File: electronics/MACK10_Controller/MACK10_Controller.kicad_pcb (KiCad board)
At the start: 2 copper layers, 97.4 x 100.5 mm, 31 parts, among them J1 Stepper Motor, J10 I/O, J3 Load Cell, J4 24V IN, J5 SSD1306, J6 INPUT, J7 E_STOP, J8 LIM_TOP, J9 LIM_BOT, U1 U1 ESP32_DEVKIT_30P, U2 HX711, U3 TMC2208, U4 LM2596 Buck Converter

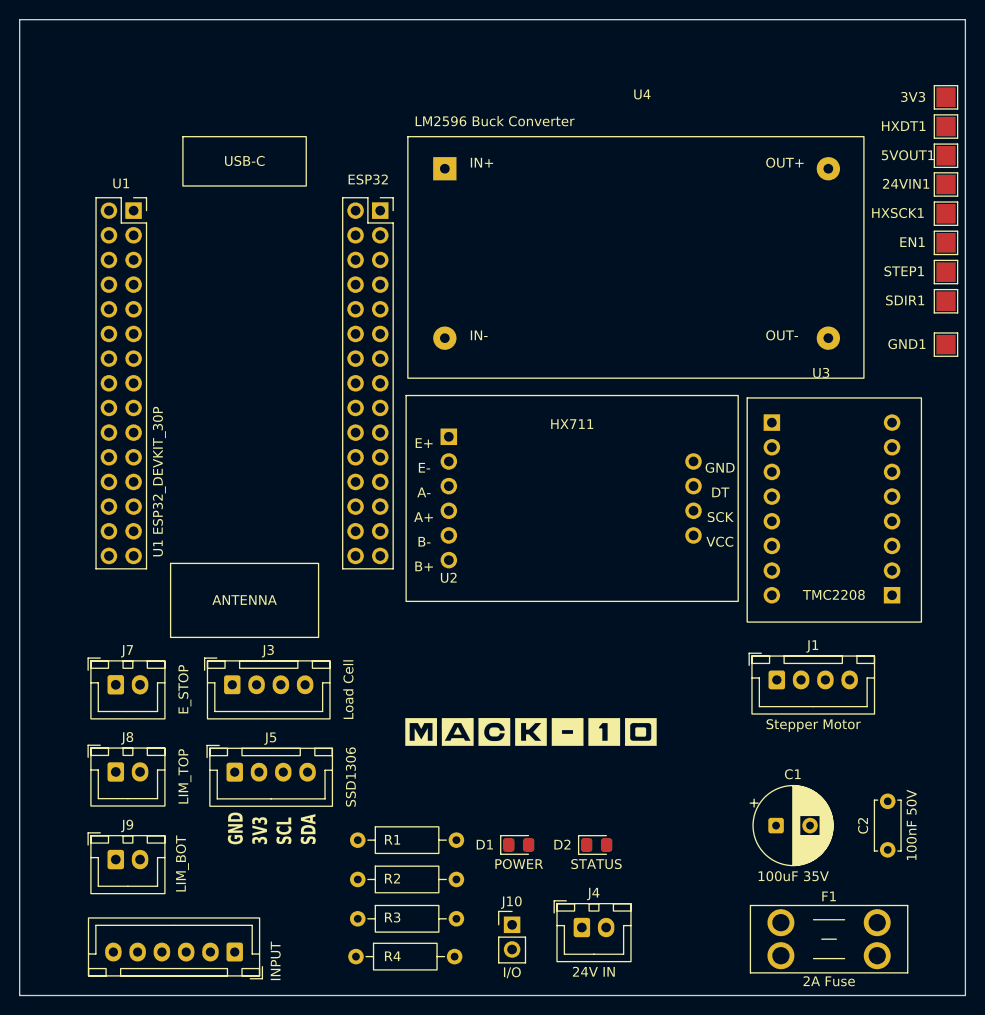
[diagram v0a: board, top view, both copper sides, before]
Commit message: Add Todo and various PCB updates
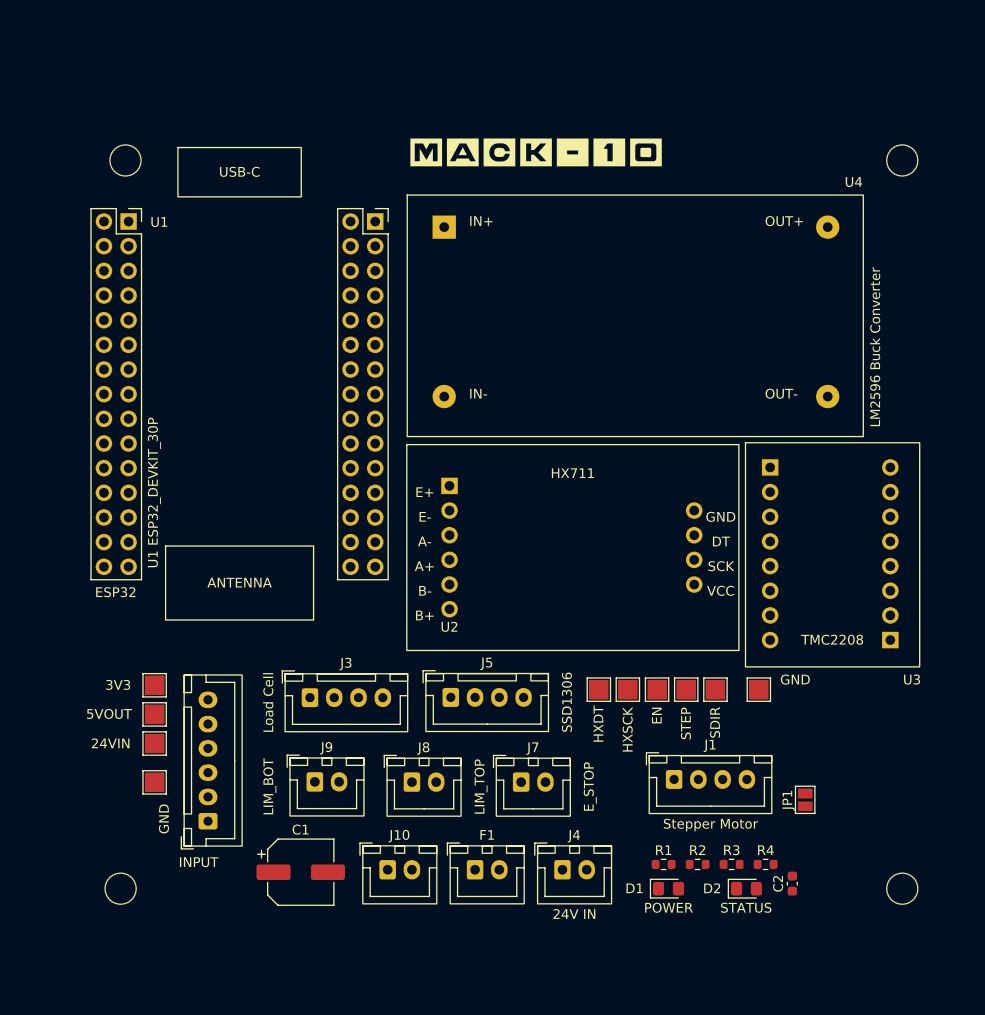
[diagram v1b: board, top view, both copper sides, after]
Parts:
- added JP1: FUSE_BYPASS, Jumper:SolderJumper-2_P1.3mm_Open_Pad1.0x1.5mm, F.Cu at (95.0, 90.8)
- added REF**: MountingHole_3.2mm_M3, MountingHole:MountingHole_3.2mm_M3, F.Cu at (25.0, 25.0)
- added REF**: MountingHole_3.2mm_M3, MountingHole:MountingHole_3.2mm_M3, F.Cu at (105.0, 100.0)
- added REF**: MountingHole_3.2mm_M3, MountingHole:MountingHole_3.2mm_M3, F.Cu at (105.0, 25.0)
- added REF**: MountingHole_3.2mm_M3, MountingHole:MountingHole_3.2mm_M3, F.Cu at (24.5, 100.0)
- added TP4: GND, TestPoint:TestPoint_Pad_2.0x2.0mm, F.Cu at (28.0, 89.0)
- C1: footprint Capacitor_THT:CP_Radial_D8.0mm_P3.50mm -> Capacitor_SMD:CP_Elec_6.3x5.4
- C2: footprint Capacitor_THT:C_Disc_D5.0mm_W2.5mm_P5.00mm -> Capacitor_SMD:C_0603_1608Metric
- F1: footprint Fuse:Fuseholder_Blade_Mini_Keystone_3568 -> Connector_JST:JST_XH_B2B-XH-A_1x02_P2.50mm_Vertical
- J10: footprint Connector_PinHeader_2.54mm:PinHeader_1x02_P2.54mm_Vertical -> Connector_JST:JST_XH_B2B-XH-A_1x02_P2.50mm_Vertical
- R1, R2, R3, R4: footprint Resistor_THT:R_Axial_DIN0207_L6.3mm_D2.5mm_P10.16mm_Horizontal -> Resistor_SMD:R_0603_1608Metric
- TP1: renamed from 3V3; value TP1 -> 3V3
- TP2: renamed from HXDT1; value TP2 -> HXDT
- TP3: renamed from 5VOUT1; value TP3 -> 5VOUT
- TP4: renamed from GND1; value TP4 -> GND
- TP5: renamed from 24VIN1; value TP5 -> 24VIN
- TP6: renamed from HXSCK1; value TP6 -> HXSCK
- TP7: renamed from EN1; value TP7 -> EN
- TP8: renamed from STEP1; value TP8 -> STEP
- TP9: renamed from SDIR1; value TP9 -> SDIR
- moved TP1 101.5 mm to (28.0, 79.0)
- moved TP5 99.8 mm to (28.0, 85.0)
- moved TP3 99.8 mm to (28.0, 82.0)
- moved TP2 68.1 mm to (73.8, 79.5), turned to 90 degrees
- moved TP6 59.0 mm to (76.7, 79.5), turned to 90 degrees
- moved TP7 54.8 mm to (79.7, 79.5), turned to 90 degrees
- moved TP8 50.6 mm to (82.8, 79.5), turned to 90 degrees
- moved C1 49.2 mm to (43.0, 98.3)
- moved TP9 46.5 mm to (85.8, 79.5), turned to 90 degrees
- moved R4 43.2 mm to (90.9, 97.5)
- moved J7 42.9 mm to (65.8, 89.0)
- moved TP4 40.4 mm to (90.2, 79.5), turned to 90 degrees
- moved R3 38.9 mm to (87.4, 97.5)
- moved R2 35.0 mm to (83.9, 97.5)
- moved F1 32.0 mm to (61.0, 98.0)
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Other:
- board outline removed
- board text removed: "3V3"
- board text removed: "GND"
- board text removed: "SCL"
- board text removed: "SDA"
